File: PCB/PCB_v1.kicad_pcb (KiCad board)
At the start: 2 copper layers, 50 x 40 mm, 9 parts, among them J1 Accelerometer, J2 Flysky FS2A Receiver, J3 DC-DC, J4 Battery Left, J5 Battery Right, J6 ESC_Left, J7 ESC_Right, J8 LED, U1 Teensy4.0

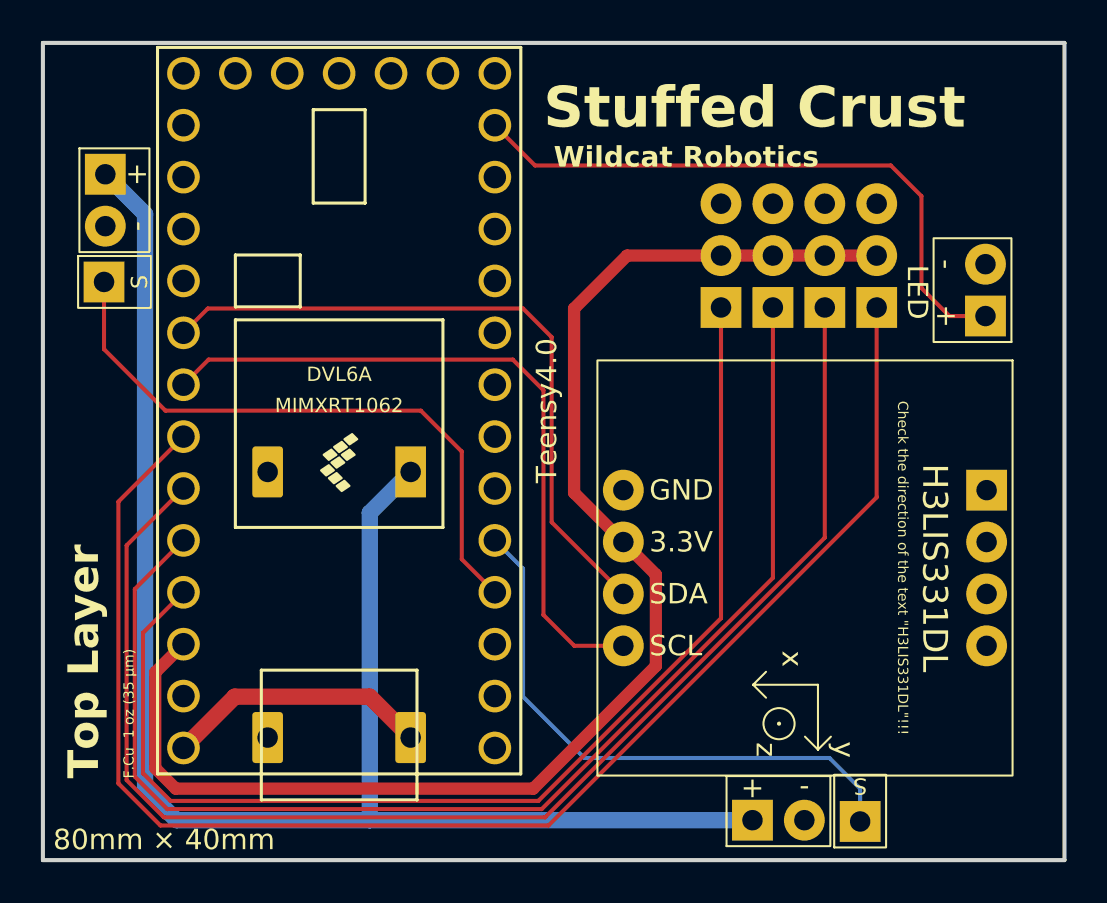
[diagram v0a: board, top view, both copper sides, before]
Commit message: Finished PCB Layout
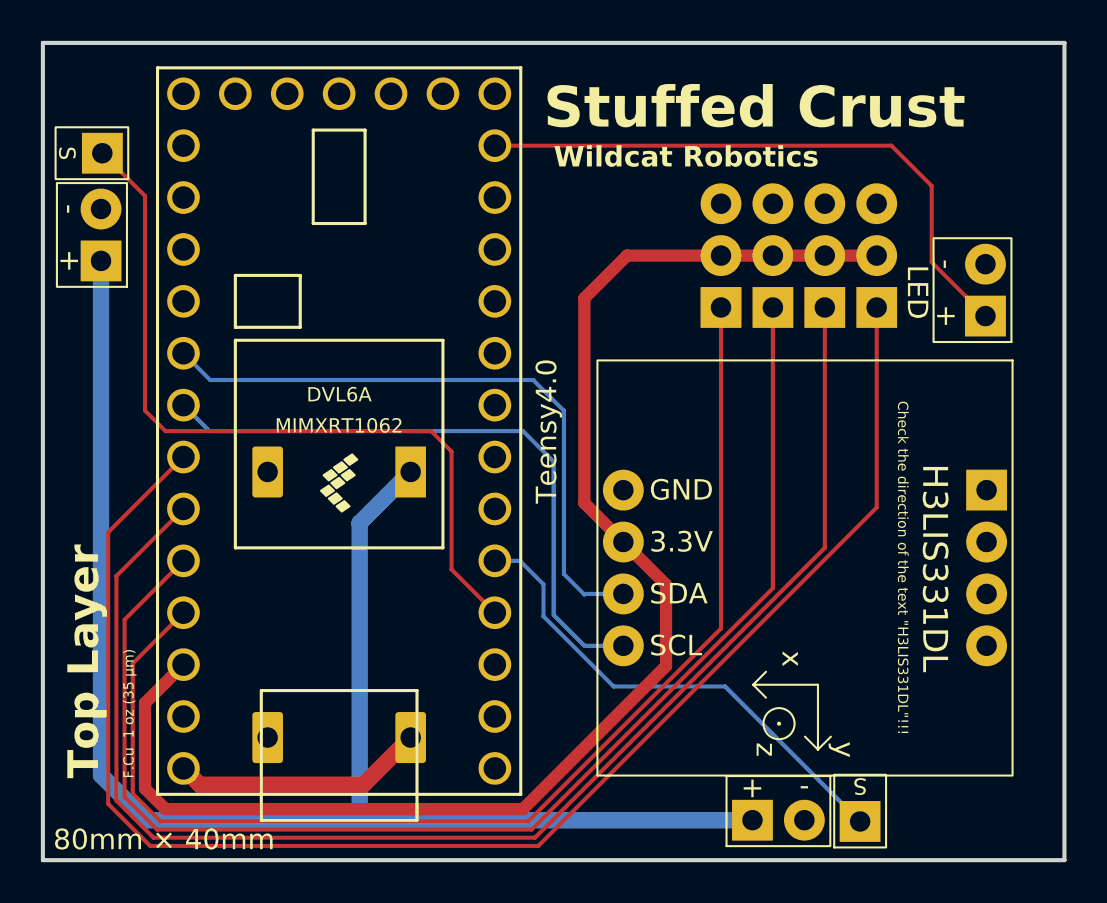
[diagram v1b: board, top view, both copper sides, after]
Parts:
- moved J4 7.17 mm to (174.1, 71.9), turned to 180 degrees
- moved J6 4.49 mm to (174.2, 66.7), turned to 180 degrees
- moved U1 1.00 mm to (184.5, 79.0)
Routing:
- net /S_ESC_Left_2: track 30.4 -> 38.1 mm
- net /S_ESC_Right_3: track 28.9 -> 24.1 mm
- net /SCL_19: track 34.3 -> 30.8 mm
- net /12V: track 79.1 -> 76.1 mm
- net /SDA_18: track 33.1 -> 31.1 mm
- net /CH4_20: track 72.2 -> 73.6 mm
- net /CH3_21: track 67.3 -> 68.7 mm
- net /CH1_23: track 57.4 -> 58.9 mm
- net /CH2_22: track 62.4 -> 63.8 mm
- net /3.3V: track 69.1 -> 70.5 mm
- net /LED: track 30.5 -> 29.7 mm
- net /5V: track 13.0 -> 12.4 mm
- added copper zone on F.Cu, net /GND
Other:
- board text added: "(Robot Center)"
